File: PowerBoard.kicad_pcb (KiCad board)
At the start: 2 copper layers, 138.9 x 105.6 mm, 15 parts, among them J101 Conn_01x04_Pin, J102 Conn_01x04_Pin, J103 Conn_01x04_Pin, J104 Conn_01x04_Pin, J105 Conn_01x02_Pin, J106 Conn_01x02_Pin, J107 Conn_01x02_Pin, J108 Conn_01x06_Pin, J109 Conn_01x06_Pin, J110 USB_C_Receptacle, U101 Teensy4.1, U103 D24V50F5, U104 2472

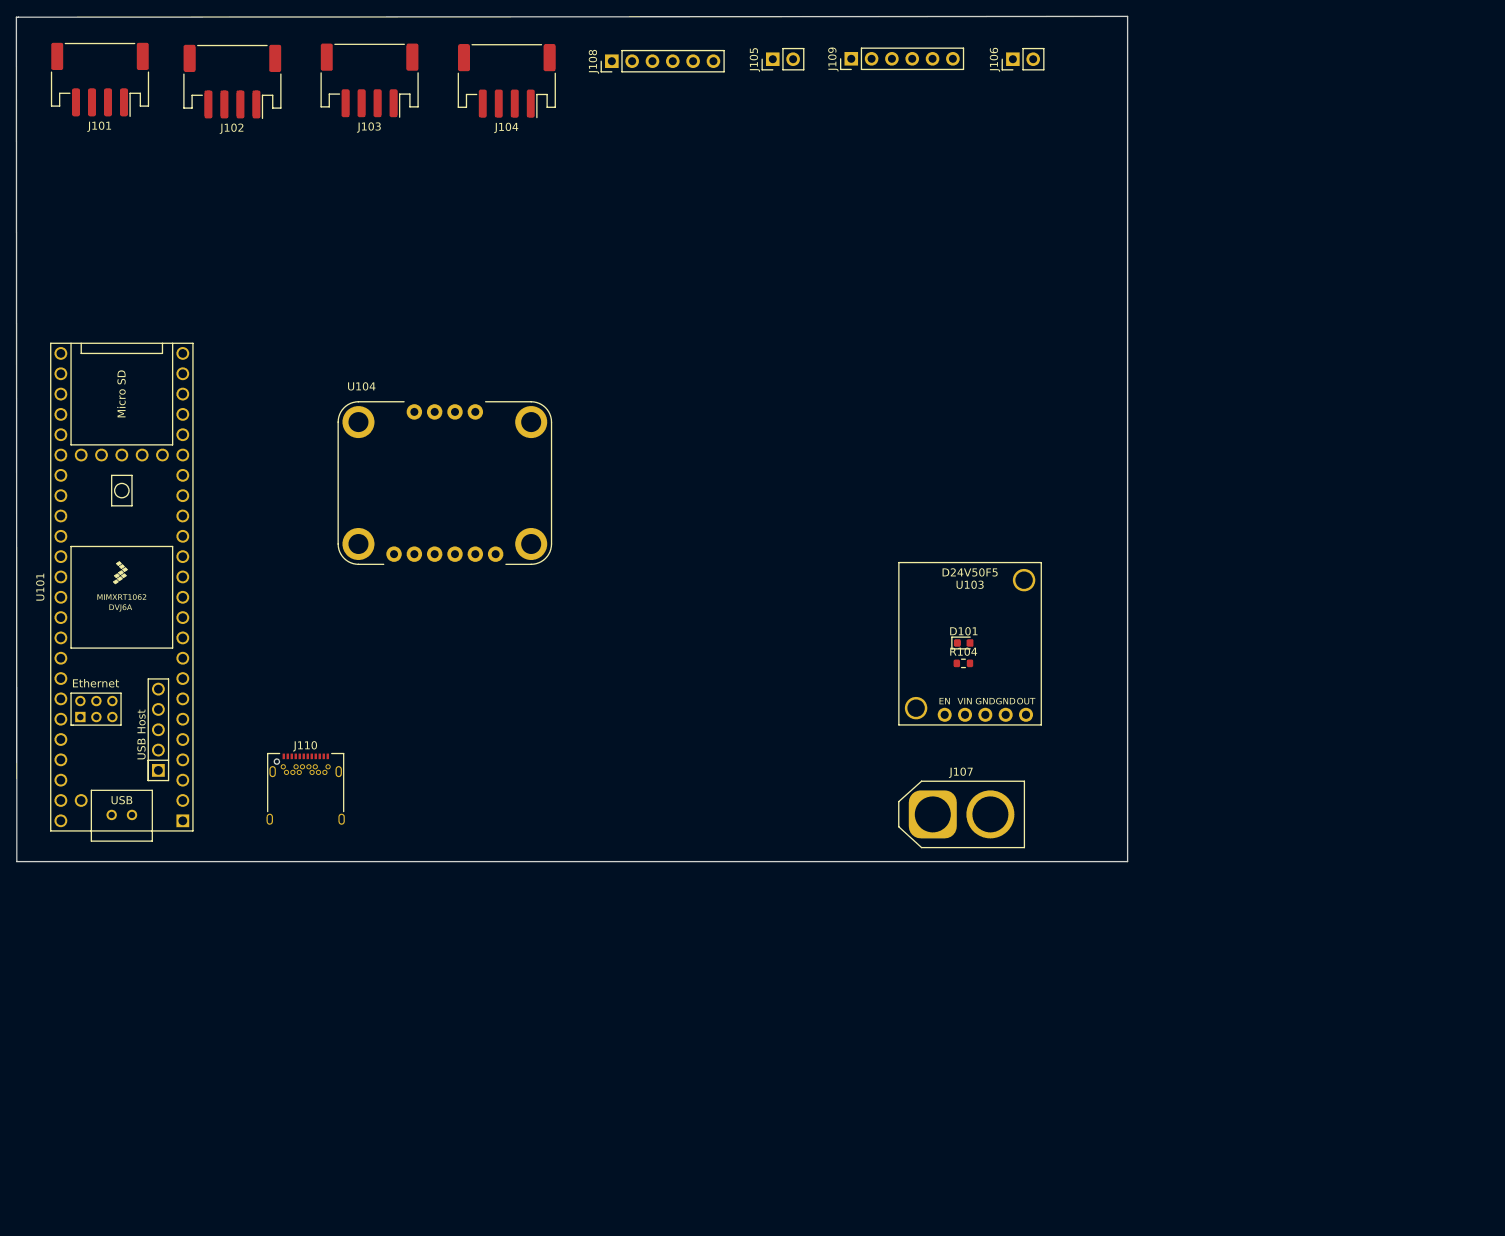
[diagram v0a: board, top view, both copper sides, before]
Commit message: weedies
weedies
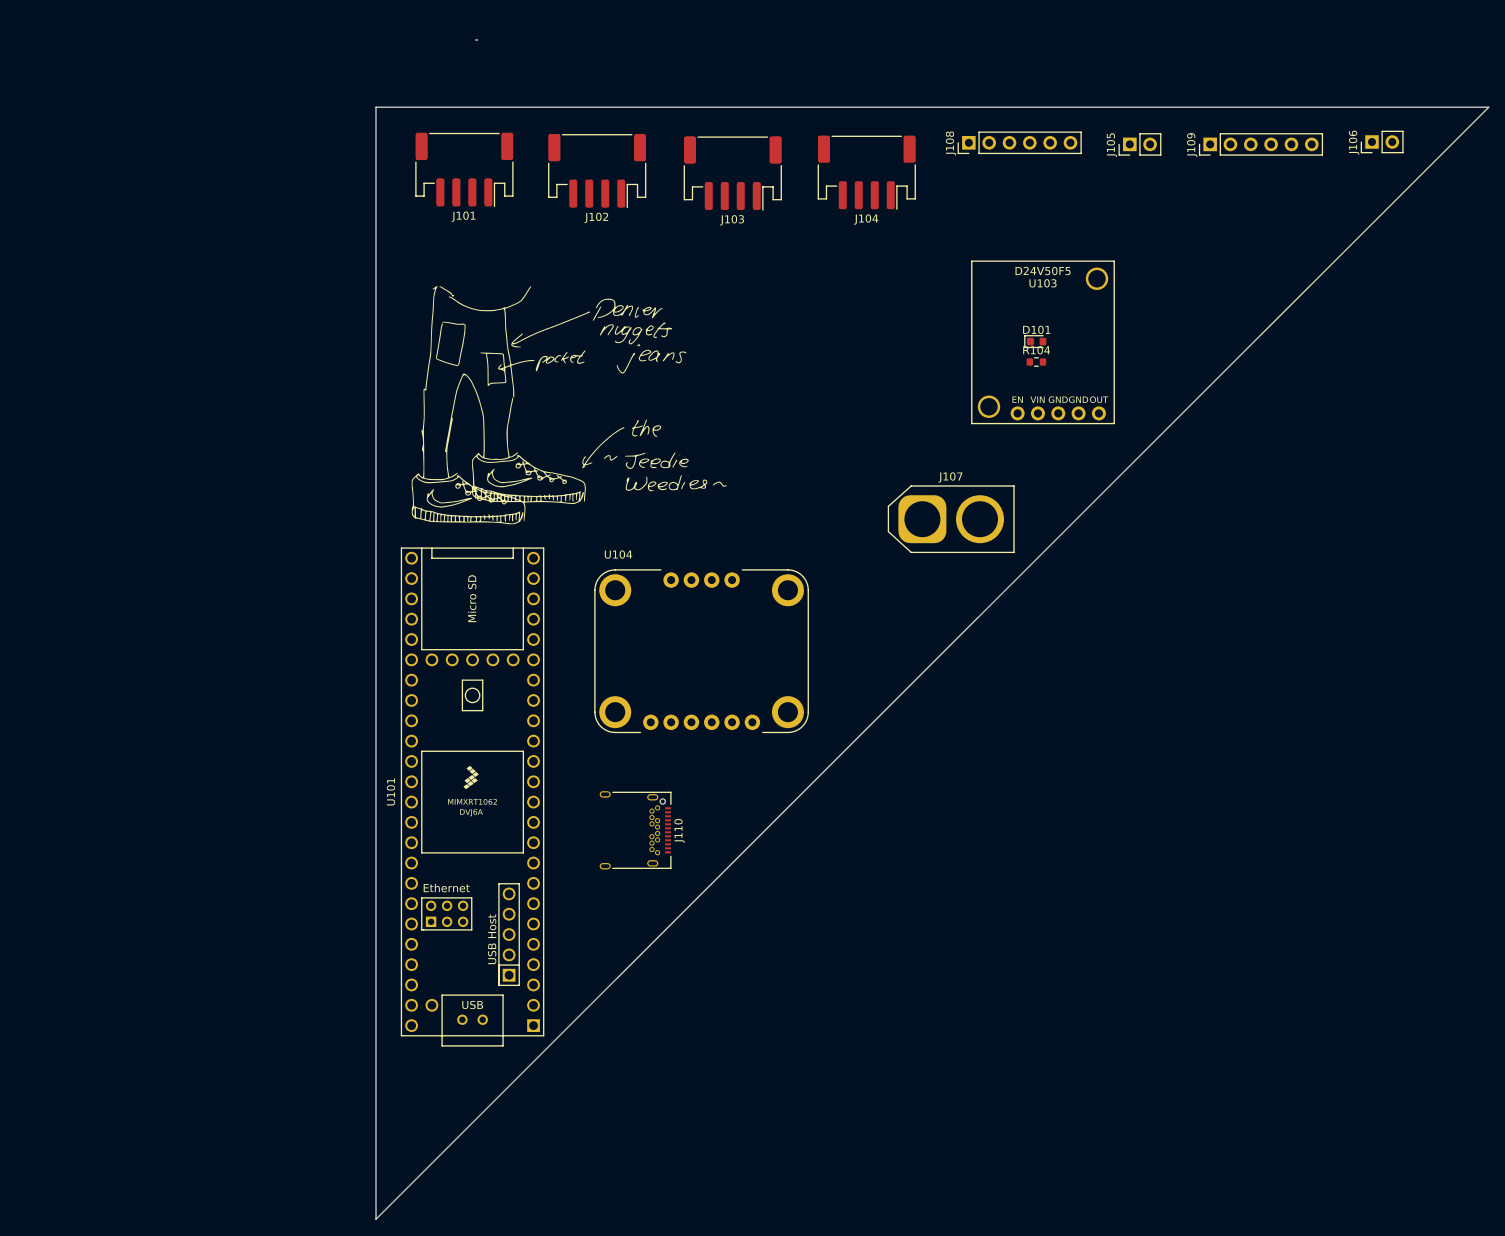
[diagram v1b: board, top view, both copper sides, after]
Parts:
- added G***: LOGO, memes:weedies2, F.Cu at (130.0, 82.4)
- moved U101 50.8 mm to (115.9, 129.7)
- moved J102 46.9 mm to (131.4, 52.1)
- moved J101 46.9 mm to (114.8, 52.0)
- moved J103 46.9 mm to (148.4, 52.4)
- moved J104 46.4 mm to (165.2, 52.3)
- moved J109 46.1 mm to (208.1, 48.8)
- moved J106 46.1 mm to (228.3, 48.5)
- moved J105 45.9 mm to (198.0, 48.8)
- moved J108 45.8 mm to (177.9, 48.6)
- moved J110 40.5 mm to (135.3, 134.5), turned to -90 degrees
- moved R104 38.8 mm to (186.3, 76.0)
- moved D101 38.8 mm to (186.4, 73.5)
- moved U103 38.8 mm to (187.2, 63.4)
- moved U104 38.4 mm to (144.5, 112.2)
- moved J107 36.9 mm to (172.1, 95.7)
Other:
- board size 138.9 x 105.6 mm -> 139.1 x 147.4 mm
